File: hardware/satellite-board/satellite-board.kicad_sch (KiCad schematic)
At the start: 27 parts, among them J1 MTJ-88ARX1-FSM-LG, J2 B2B-PH-K-S, Q1 2N7002, U1 LORA1262-915TCXO, U2 XC6220B331MR, U3 ESP32-C6-DEVKITC-1-N8, U4 MAX3485

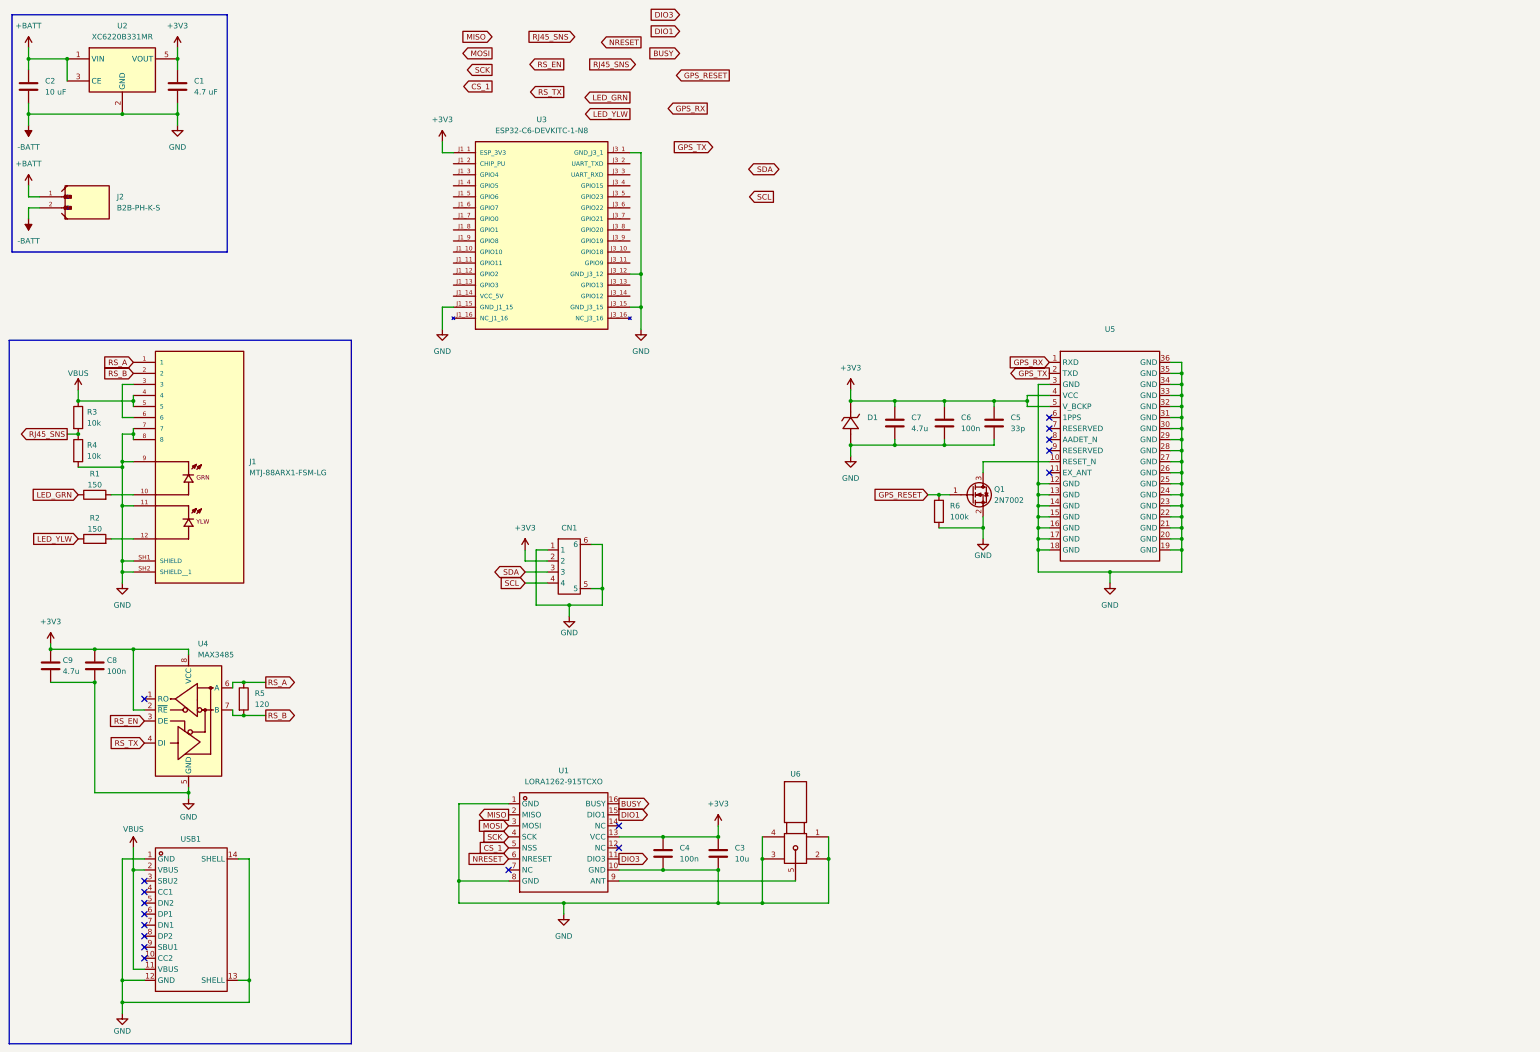
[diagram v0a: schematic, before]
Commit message: Satelite Schematic Finished
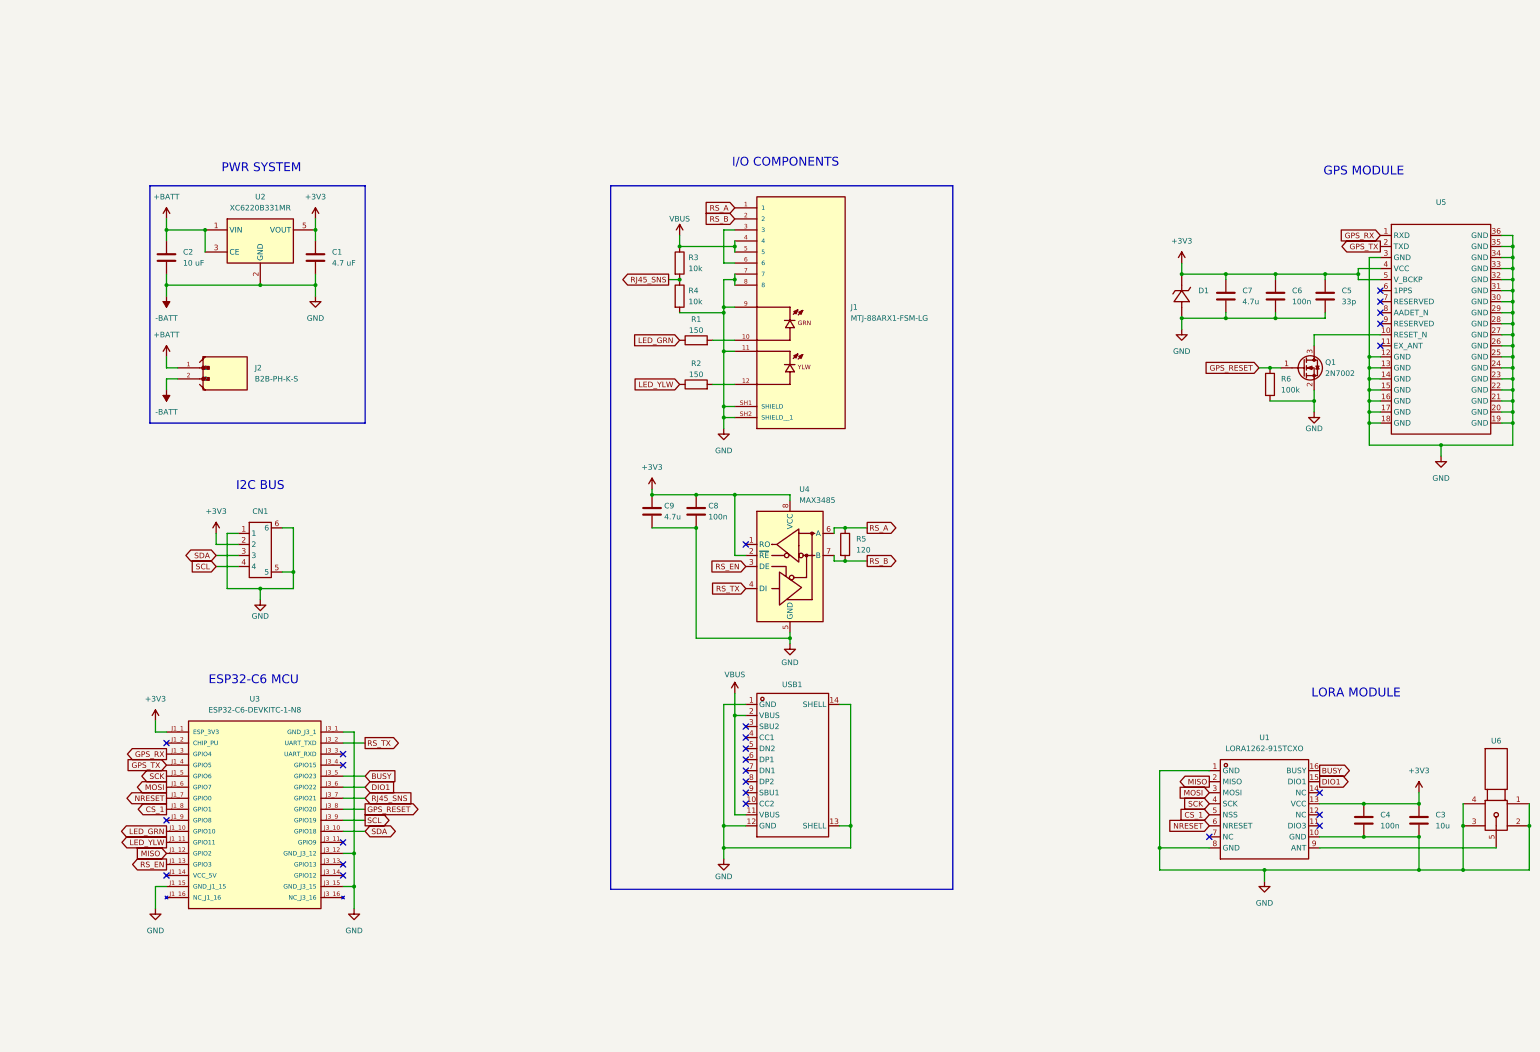
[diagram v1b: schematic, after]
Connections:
- net BUSY: now also U3.J3_5 (GPIO23)
- net CS_1: now also U3.J1_8 (GPIO1)
- net DIO1: now also U3.J3_6 (GPIO22)
- net GPS_RESET: now also U3.J3_8 (GPIO20)
- net GPS_RX: now also U3.J1_3 (GPIO4)
- net GPS_TX: now also U3.J1_4 (GPIO5)
- net LED_GRN: now also U3.J1_10 (GPIO10)
- net LED_YLW: now also U3.J1_11 (GPIO11)
- net MISO: now also U3.J1_12 (GPIO2)
- net MOSI: now also U3.J1_6 (GPIO7)
- net NRESET: now also U3.J1_7 (GPIO0)
- net RJ45_SNS: now also U3.J3_7 (GPIO21)
- net RS_EN: now also U3.J1_13 (GPIO3)
- net RS_TX: now also U3.J3_2 (UART_TXD)
- net SCK: now also U3.J1_5 (GPIO6)
- net SCL: now also U3.J3_9 (GPIO19)
- net SDA: now also U3.J3_10 (GPIO18)
- net DIO3: no longer names the net of U1.11 (DIO3)
- no-connect marks 17 -> 26
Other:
- note added: "ESP32-C6 MCU"
- note added: "GPS MODULE"
- note added: "I/O COMPONENTS"
- note added: "I2C BUS"
- note added: "LORA MODULE"
- note added: "PWR SYSTEM"
- moved on the sheet: C1, C2, C3, C4, C5, C6, C7, C8, C9, CN1, D1, J1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
